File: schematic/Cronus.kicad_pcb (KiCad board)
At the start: 2 copper layers, 70 x 50 mm, 16 parts, among them J1 5V_In, J2 DCL, J3 DCS, J4 DD0, J5 LS1, J6 LS2, J7 GND, U1 ESP32, U2 DS3231

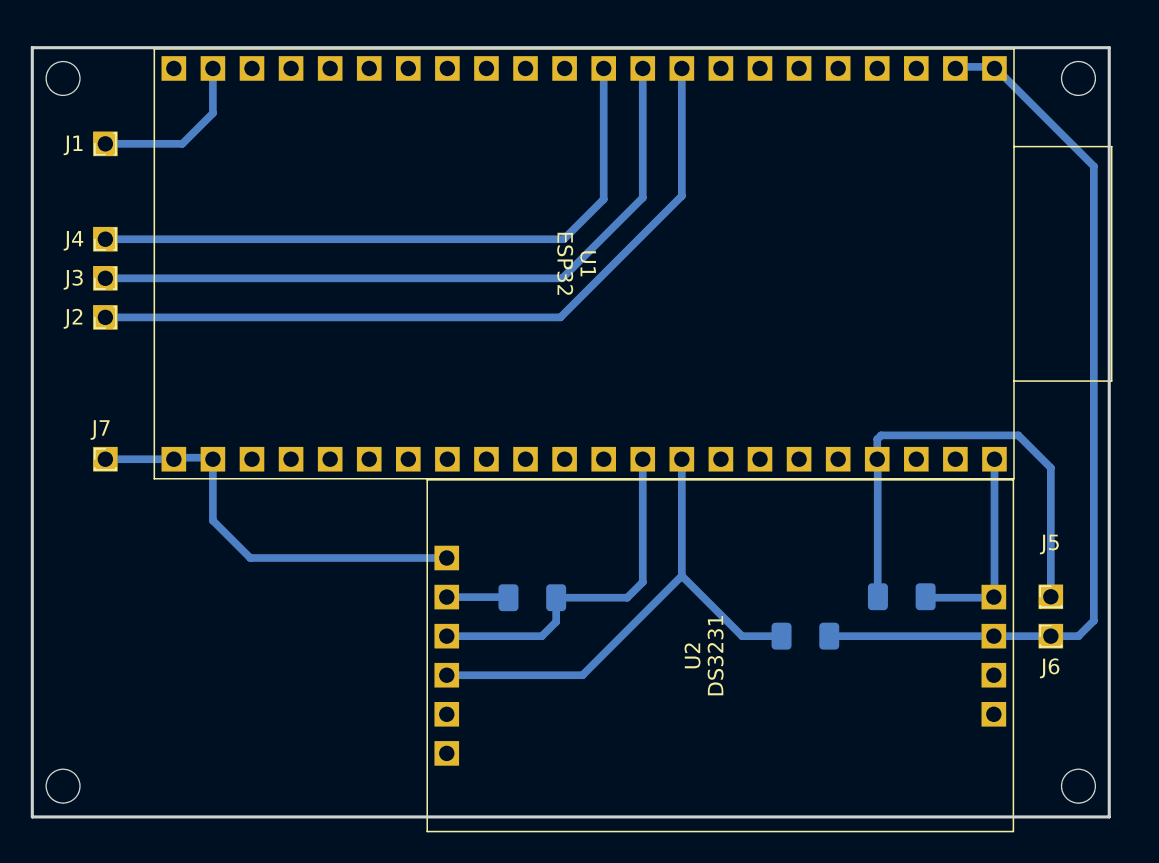
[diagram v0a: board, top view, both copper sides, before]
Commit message: Remake schematic with KiCad #3
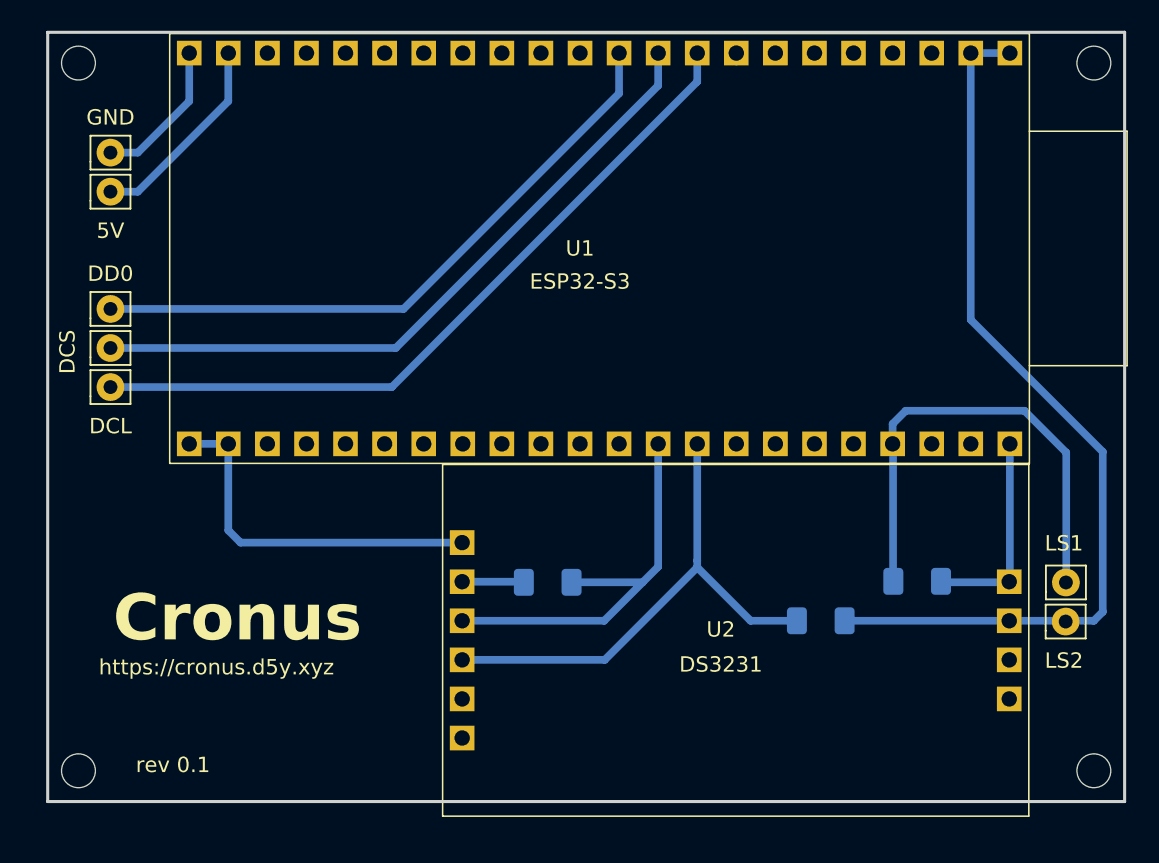
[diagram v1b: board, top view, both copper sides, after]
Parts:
- removed REF** (x4): MountingHole_2.2mm_M2, MountingHole:MountingHole_2.2mm_M2
- added H1: MountingHole, MountingHole:MountingHole_2.2mm_M2, F.Cu at (108.5, 64.8)
- added H2: MountingHole, MountingHole:MountingHole_2.2mm_M2, F.Cu at (174.5, 64.8)
- added H3: MountingHole, MountingHole:MountingHole_2.2mm_M2, F.Cu at (108.5, 110.8)
- added H4: MountingHole, MountingHole:MountingHole_2.2mm_M2, F.Cu at (174.5, 110.8)
- J1: value 5V_In -> GND; footprint Connector_PinHeader_1.00mm:PinHeader_1x01_P1.00mm_Vertical -> Connector_Pin:Pin_D0.9mm_L10.0mm_W2.4mm_FlatFork
- J2: value DCL -> 5V; footprint Connector_PinHeader_1.00mm:PinHeader_1x01_P1.00mm_Vertical -> Connector_Pin:Pin_D0.9mm_L10.0mm_W2.4mm_FlatFork
- J3: value DCS -> DCL; footprint Connector_PinHeader_1.00mm:PinHeader_1x01_P1.00mm_Vertical -> Connector_Pin:Pin_D0.9mm_L10.0mm_W2.4mm_FlatFork
- J4: value DD0 -> DCS; footprint Connector_PinHeader_1.00mm:PinHeader_1x01_P1.00mm_Vertical -> Connector_Pin:Pin_D0.9mm_L10.0mm_W2.4mm_FlatFork
- J5: value LS1 -> DD0; footprint Connector_PinHeader_1.00mm:PinHeader_1x01_P1.00mm_Vertical -> Connector_Pin:Pin_D0.9mm_L10.0mm_W2.4mm_FlatFork
- J6: value LS2 -> LS1; footprint Connector_PinHeader_1.00mm:PinHeader_1x01_P1.00mm_Vertical -> Connector_Pin:Pin_D0.9mm_L10.0mm_W2.4mm_FlatFork
- J7: value GND -> LS2; footprint Connector_PinHeader_1.00mm:PinHeader_1x01_P1.00mm_Vertical -> Connector_Pin:Pin_D0.9mm_L10.0mm_W2.4mm_FlatFork
- U1: value ESP32 -> ESP32-S3
- moved J5 63.9 mm to (110.6, 80.7)
- moved J7 63.3 mm to (172.7, 101.0)
- moved J2 8.18 mm to (110.6, 73.1), turned to 0 degrees
- moved J4 7.08 mm to (110.6, 83.3), turned to 0 degrees
- moved J3 7.08 mm to (110.6, 85.8), turned to 0 degrees
- moved J6 3.62 mm to (172.7, 98.5)
- moved R1 1.41 mm to (156.8, 101.0)
- moved R2 1.41 mm to (139.0, 98.5)
- moved R3 1.41 mm to (163.0, 98.4)
- moved U1 1.41 mm to (141.1, 76.8)
- moved U2 1.41 mm to (149.9, 102.3)
- moved J1 0.66 mm to (110.6, 70.6), turned to 0 degrees
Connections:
- J1 pad 1: +5V -> GND
- J2 pad 1: Net-(J2-Pin_1) -> +5V
- J7 pad 1: GND -> Net-(J7-Pin_1)
- R1 pad 1: Net-(J6-Pin_1) -> Net-(J7-Pin_1)
- R2 pad 1: Net-(J6-Pin_1) -> Net-(J7-Pin_1)
- R3 pad 1: Net-(J5-Pin_1) -> Net-(J6-Pin_1)
- U1 pad 1: Net-(J6-Pin_1) -> Net-(J7-Pin_1)
- U1 pad 10: Net-(J3-Pin_1) -> Net-(J4-Pin_1)
- U1 pad 11: Net-(J4-Pin_1) -> Net-(J5-Pin_1)
- U1 pad 41: Net-(J5-Pin_1) -> Net-(J6-Pin_1)
- U1 pad 9: Net-(J2-Pin_1) -> Net-(J3-Pin_1)
- U2 pad 2: Net-(J6-Pin_1) -> Net-(J7-Pin_1)
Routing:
- net Net-(J7-Pin_1): track 0.00 -> 63.6 mm
- net Net-(J2-Pin_1): track 49.1 -> 0.00 mm
- net Net-(J6-Pin_1): track 62.9 -> 31.4 mm
- net Net-(J5-Pin_1): track 31.0 -> 41.5 mm
- net GND: track 40.8 -> 47.0 mm
- net Net-(U1-GPIO38): track 23.1 -> 26.8 mm
- net Net-(J4-Pin_1): track 42.1 -> 44.8 mm
- net Net-(J3-Pin_1): track 45.6 -> 48.2 mm
- net +5V: track 10.8 -> 13.2 mm
- net unconnected-(U1-GPIO15-Pad8): track 0.00 -> 0.56 mm
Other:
- board text added: "Cronus"
- board text added: "https://cronus.d5y.xyz"
- board text added: "rev 0.1"
